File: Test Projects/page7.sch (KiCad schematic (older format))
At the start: 57 parts, among them P2 CONN_01X03, P30 CONN_01X03, P38 CONN_01X06, P39 CONN_01X06, P64 DIN1, P65 DOUT1, P66 SDA0, P67 SCL0, P68 MCLK, P69 BCLK, P70 LRCLK, P71 DIN0, P72 DOUT0, U31 SGTL5000, U5 SGTL5000

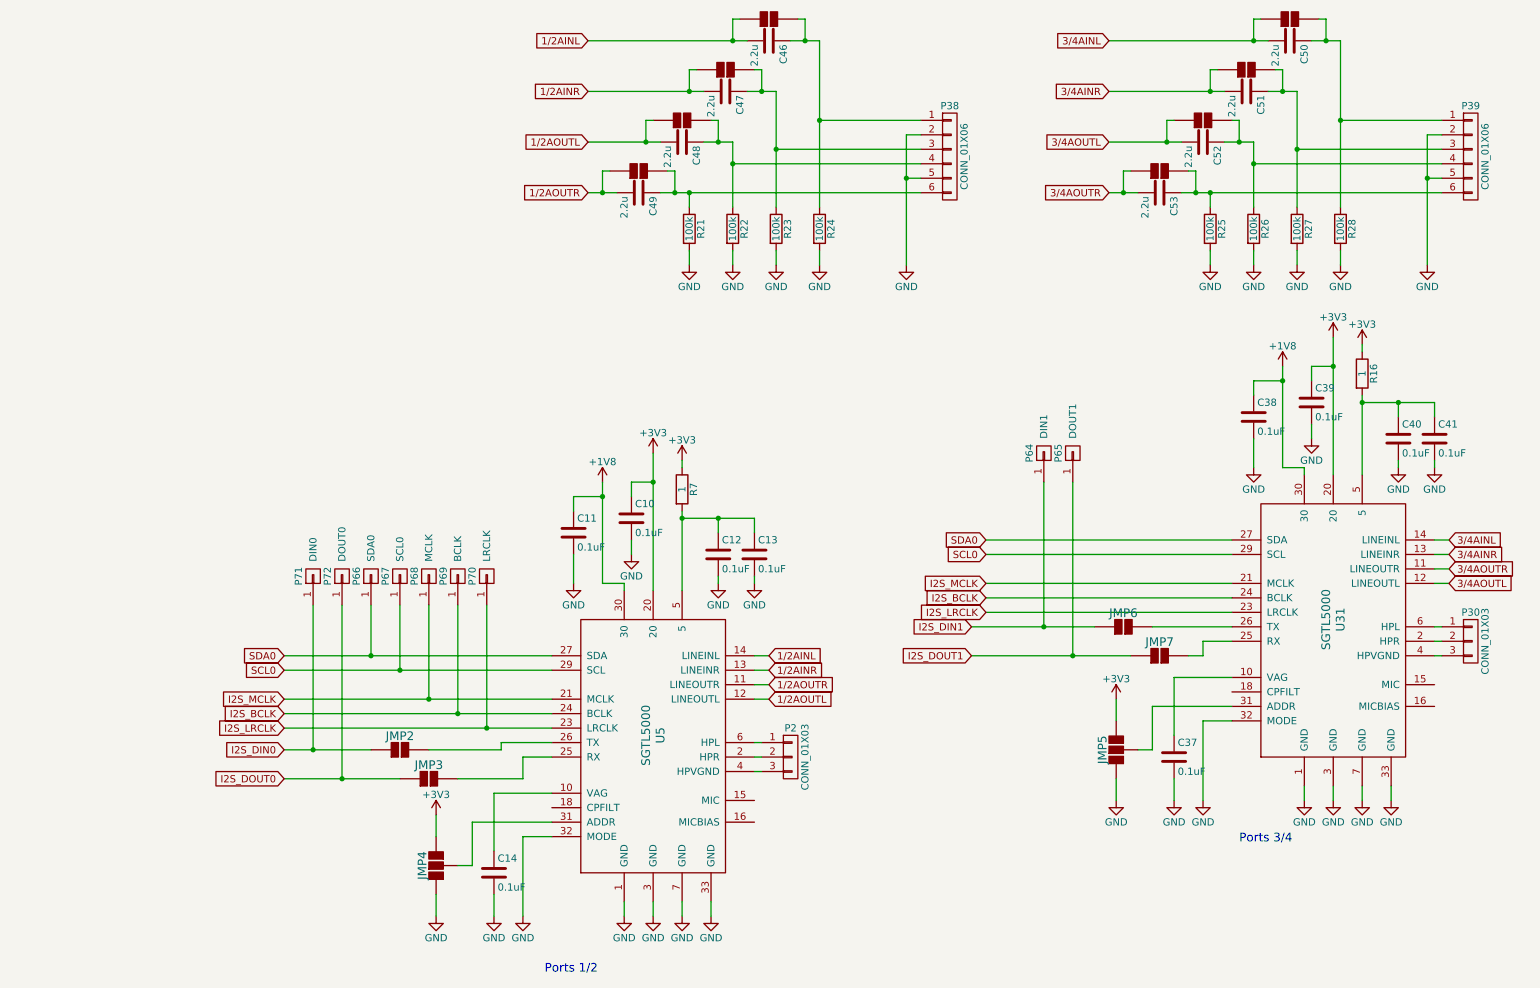
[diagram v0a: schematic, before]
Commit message: moar layout
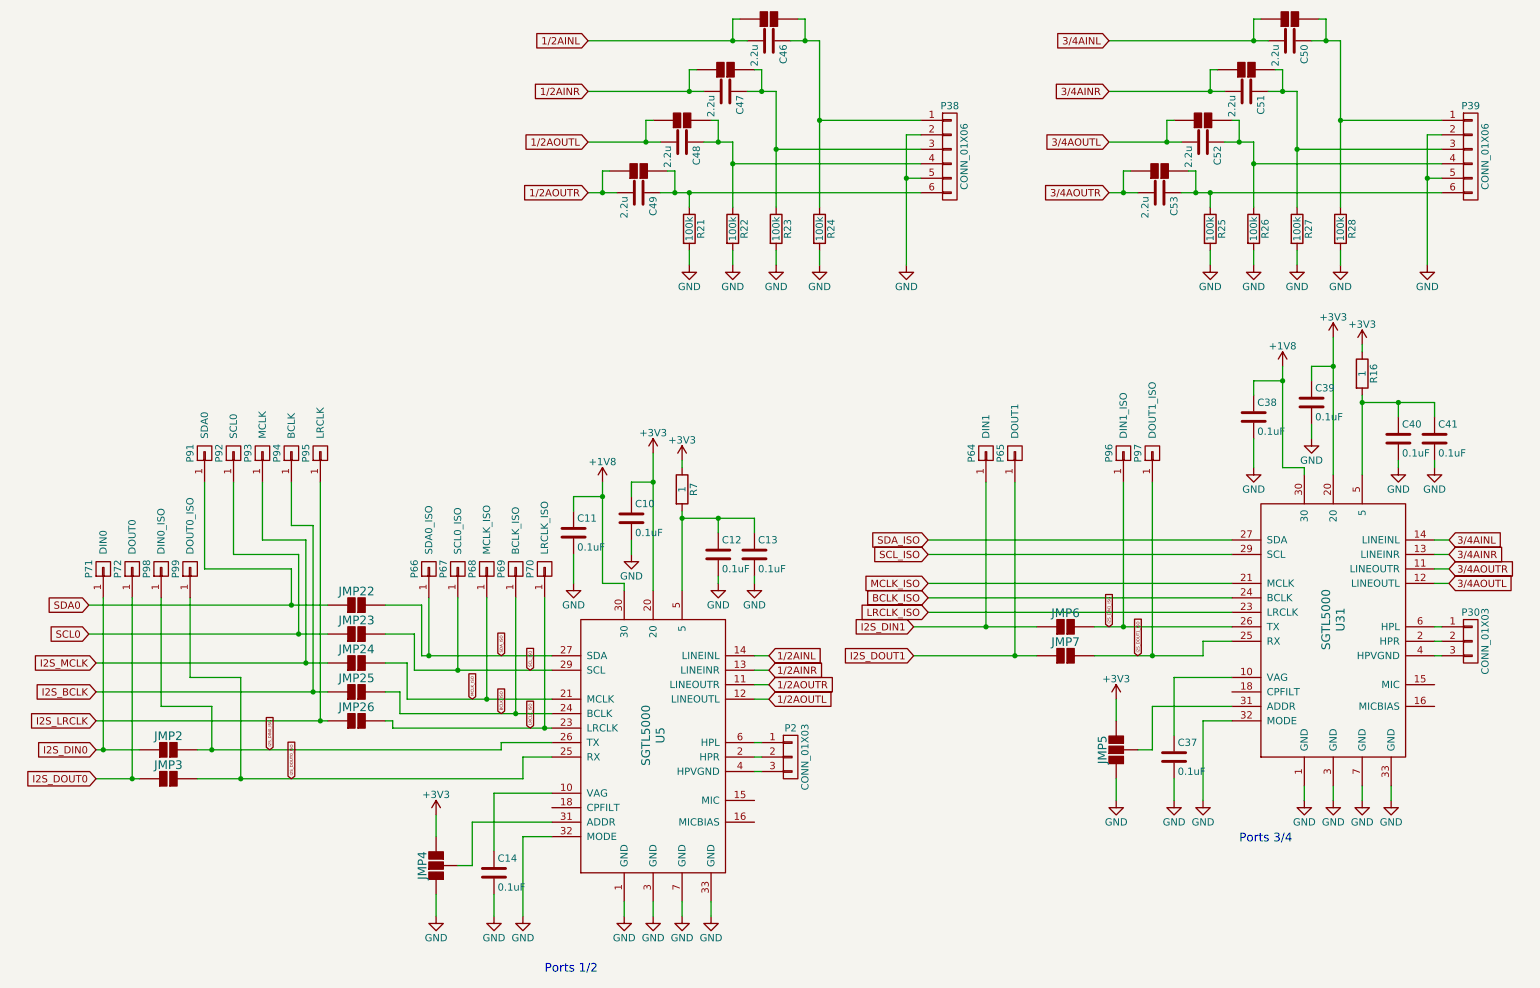
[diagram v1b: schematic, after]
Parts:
- added JMP22, JMP23, JMP24, JMP25, JMP26: 2Jumper, SparkFun-Footprints:SF-2way-open, symbol 2Jumper
- added P91: SDA0, SparkFun-Footprints:TestHole, symbol CONN_01X01
- added P92: SCL0, SparkFun-Footprints:TestHole, symbol CONN_01X01
- added P93: MCLK, SparkFun-Footprints:TestHole, symbol CONN_01X01
- added P94: BCLK, SparkFun-Footprints:TestHole, symbol CONN_01X01
- added P95: LRCLK, SparkFun-Footprints:TestHole, symbol CONN_01X01
- added P96: DIN1_ISO, SparkFun-Footprints:TestHole, symbol CONN_01X01
- added P97: DOUT1_ISO, SparkFun-Footprints:TestHole, symbol CONN_01X01
- added P98: DIN0_ISO, SparkFun-Footprints:TestHole, symbol CONN_01X01
- added P99: DOUT0_ISO, SparkFun-Footprints:TestHole, symbol CONN_01X01
- P66: value SDA0 -> SDA0_ISO
- P67: value SCL0 -> SCL0_ISO
- P68: value MCLK -> MCLK_ISO
- P69: value BCLK -> BCLK_ISO
- P70: value LRCLK -> LRCLK_ISO
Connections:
- net I2S_BCLK: now also JMP25.1, P94.1 (P1); no longer P69.1 (P1), U31.24 (BCLK), U5.24 (BCLK)
- net I2S_LRCLK: now also JMP26.1, P95.1 (P1); no longer P70.1 (P1), U31.23 (LRCLK), U5.23 (LRCLK)
- net I2S_MCLK: now also JMP24.1, P93.1 (P1); no longer P68.1 (P1), U31.21 (MCLK), U5.21 (MCLK)
- net SCL0: now also JMP23.1, P92.1 (P1); no longer P67.1 (P1), U31.29 (SCL), U5.29 (SCL)
- net SDA0: now also JMP22.1, P91.1 (P1); no longer P66.1 (P1), U31.27 (SDA), U5.27 (SDA)
- net I2S_DOUT0_ISO: now reaches JMP3.2, U5.25 (RX)
- net I2S_DOUT0_ISO: now also P99.1 (P1)
- net I2S_DIN0_ISO: now reaches JMP2.2, U5.26 (TX)
- net I2S_DIN0_ISO: now also P98.1 (P1)
- net I2S_DOUT1_ISO: now reaches JMP7.2, U31.25 (RX)
- net I2S_DOUT1_ISO: now also P97.1 (P1)
- net I2S_DIN1_ISO: now reaches JMP6.2, U31.26 (TX)
- net I2S_DIN1_ISO: now also P96.1 (P1)
- new net BCLK_ISO: JMP25.2, P69.1 (P1), U31.24 (BCLK), U5.24 (BCLK)
- new net LRCLK_ISO: JMP26.2, P70.1 (P1), U31.23 (LRCLK), U5.23 (LRCLK)
- new net MCLK_ISO: JMP24.2, P68.1 (P1), U31.21 (MCLK), U5.21 (MCLK)
- new net SCL_ISO: JMP23.2, P67.1 (P1), U31.29 (SCL), U5.29 (SCL)
- new net SDA_ISO: JMP22.2, P66.1 (P1), U31.27 (SDA), U5.27 (SDA)
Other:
- moved on the sheet: JMP2, JMP3, JMP6, JMP7, P64, P65, P66, P67, P68, P69, P70, P71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
